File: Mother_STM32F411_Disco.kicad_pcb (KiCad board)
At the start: 2 copper layers, 200 x 200 mm, 38 parts, among them J1 SRC_Cable, J2 0, J3 0, J4 0, U1 ESP32-DEVKIT-V1

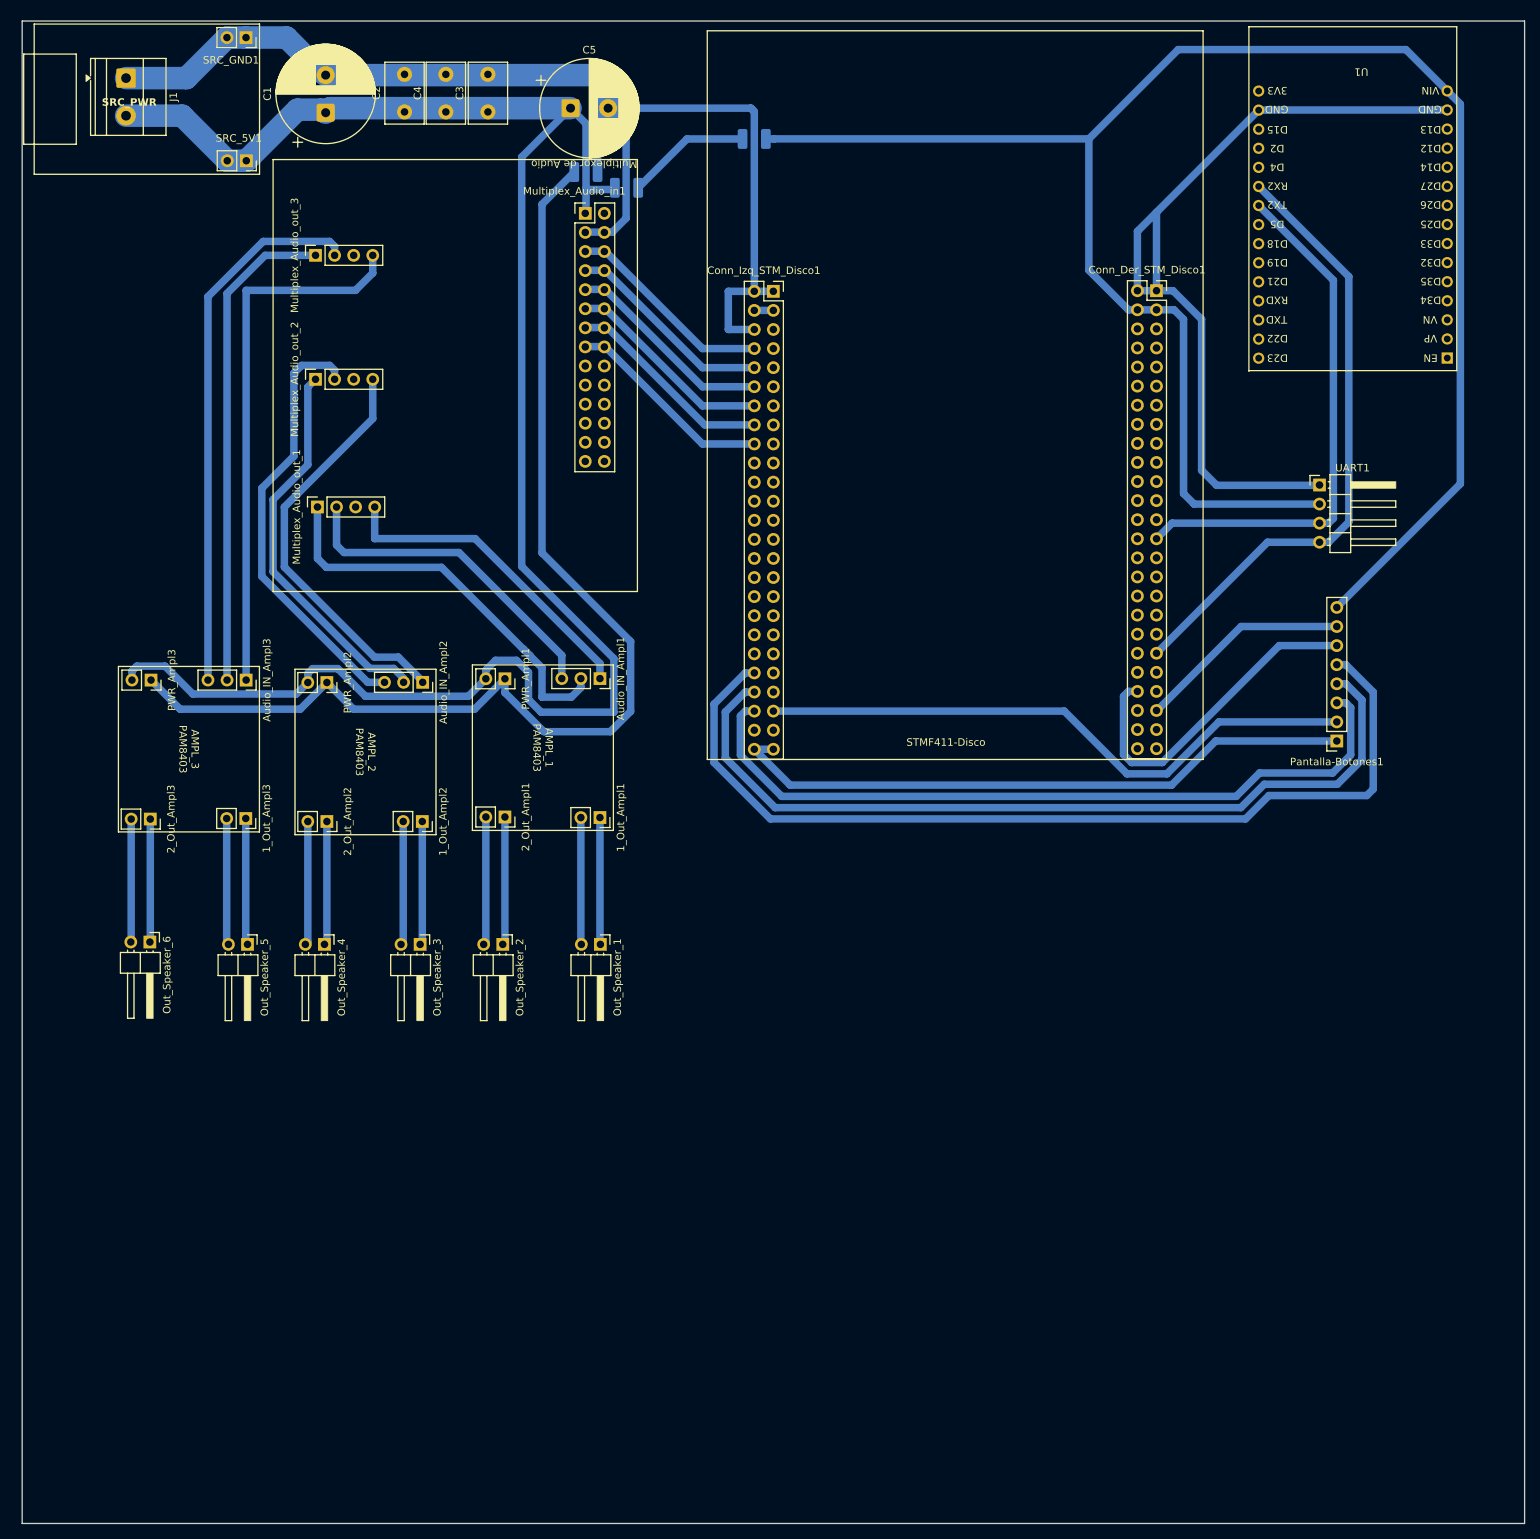
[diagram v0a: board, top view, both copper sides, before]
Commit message: PCB version 2
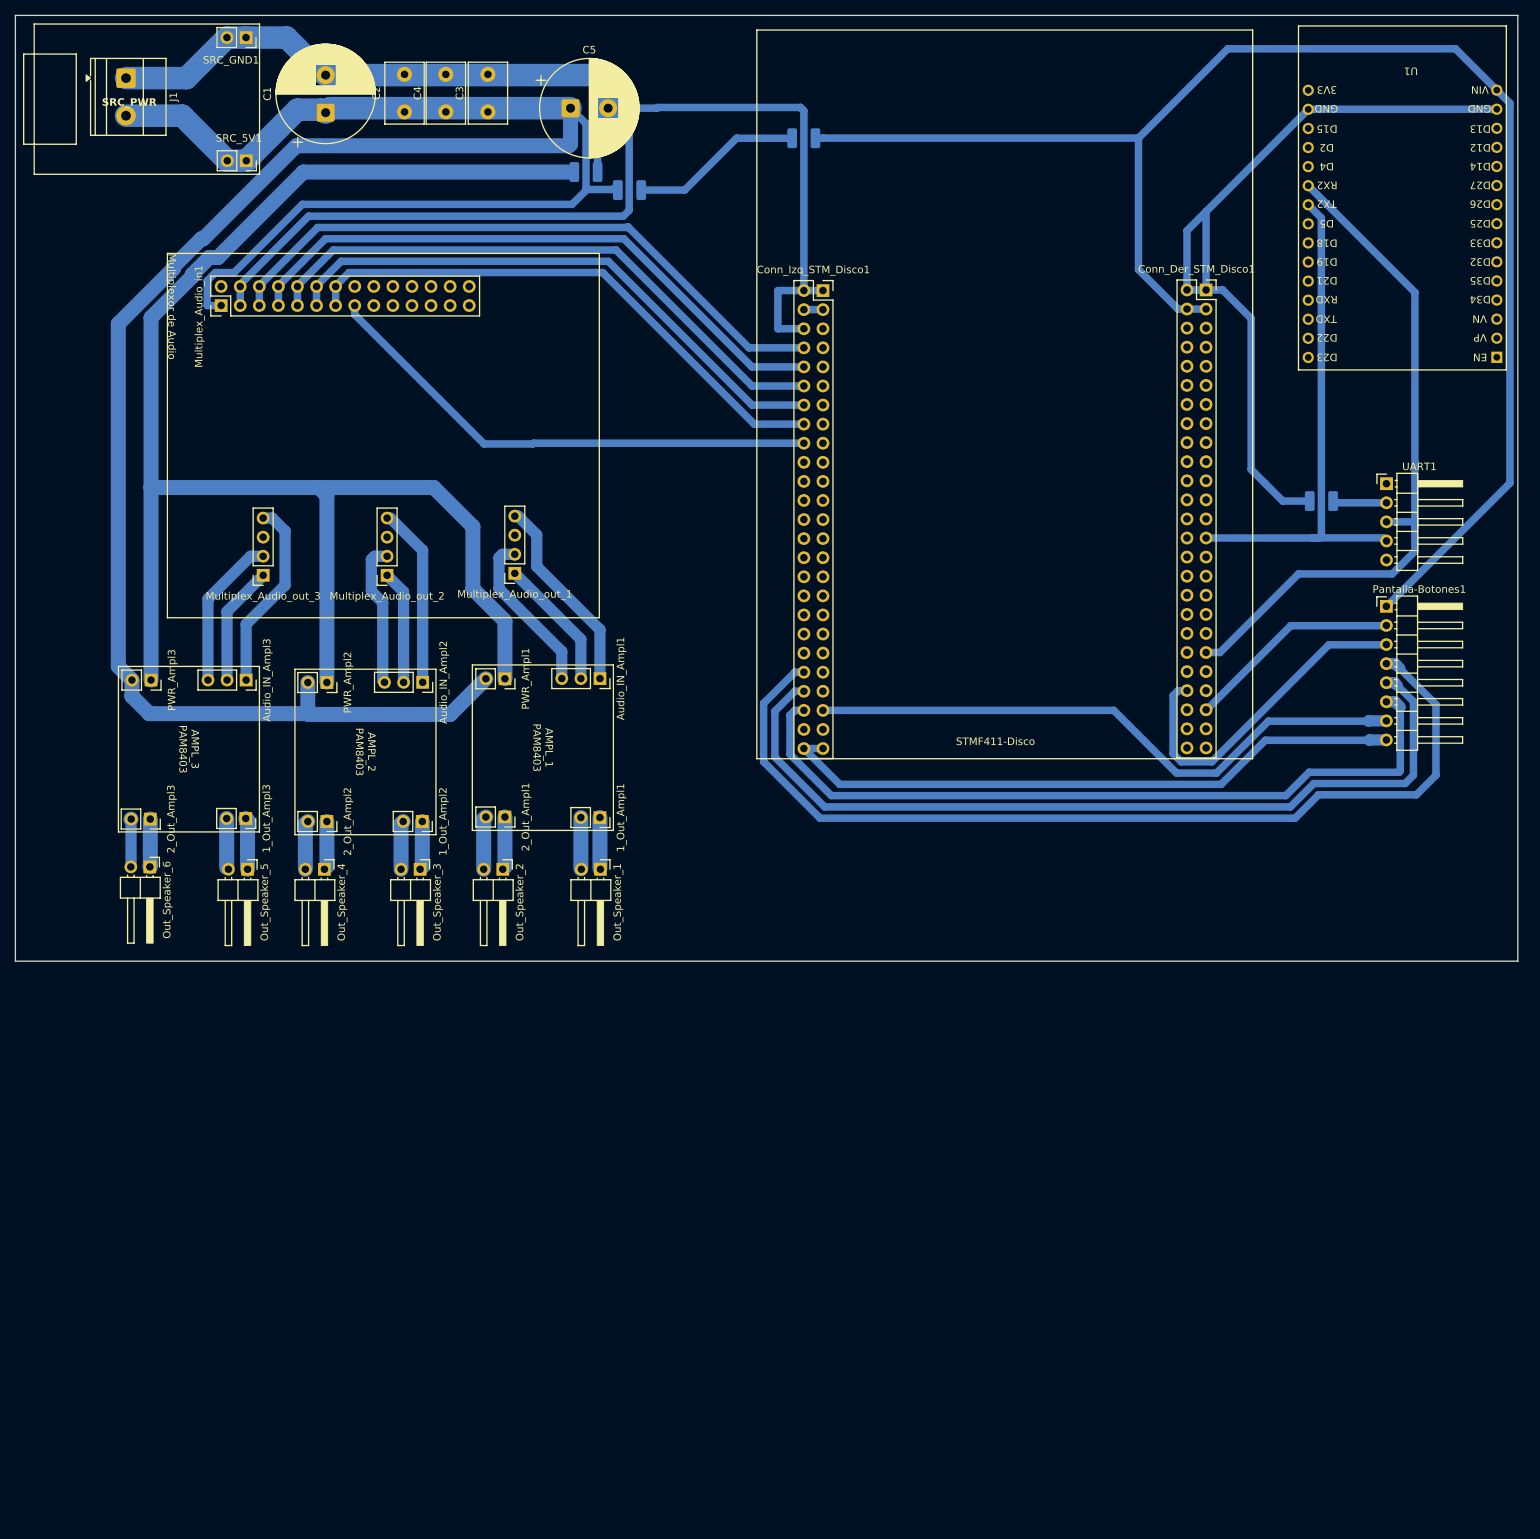
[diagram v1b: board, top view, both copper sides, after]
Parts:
- added J5: 0, Resistor_SMD:R_1210_3225Metric_Pad1.30x2.65mm_HandSolder, B.Cu at (342.9, 91.3)
- Pantalla-Botones1: footprint Connector_PinSocket_2.54mm:PinSocket_1x08_P2.54mm_Vertical -> Connector_PinHeader_2.54mm:PinHeader_1x08_P2.54mm_Horizontal
- UART1: footprint Connector_PinHeader_2.54mm:PinHeader_1x04_P2.54mm_Horizontal -> Connector_PinHeader_2.54mm:PinHeader_1x05_P2.54mm_Horizontal
- moved Multiplex_Audio_in1 50.0 mm to (196.5, 65.3), turned to 90 degrees
- moved Multiplex_Audio_out_3 43.2 mm to (202.1, 101.2), turned to 180 degrees
- moved Multiplex_Audio_out_2 27.8 mm to (218.6, 101.2), turned to 180 degrees
- moved Multiplex_Audio_out_1 27.7 mm to (235.6, 100.9), turned to 180 degrees
- moved Pantalla-Botones1 19.1 mm to (351.6, 105.3), turned to 0 degrees
- moved Out_Speaker_1 10.0 mm to (247.0, 140.3)
- moved Out_Speaker_2 10.0 mm to (234.0, 140.3)
- moved Out_Speaker_3 10.0 mm to (223.0, 140.3)
- moved Out_Speaker_4 10.0 mm to (210.2, 140.3)
- moved Out_Speaker_5 10.0 mm to (200.0, 140.3)
- moved Out_Speaker_6 10.0 mm to (187.0, 140.0)
- moved UART1 8.92 mm to (351.6, 89.0)
- moved Conn_Der_STM_Disco1 6.60 mm to (327.6, 63.2)
- moved Conn_Izq_STM_Disco1 6.60 mm to (276.6, 63.3)
- moved J2 6.60 mm to (274.1, 43.0)
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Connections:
- Pantalla-Botones1 pad 1: /GND -> /5V
- Pantalla-Botones1 pad 2: /PD14 -> /PC9
- Pantalla-Botones1 pad 3: /PD13 -> /PA8
- Pantalla-Botones1 pad 4: /PD11 -> /PD9
- Pantalla-Botones1 pad 5: /PD9 -> /PD11
- Pantalla-Botones1 pad 6: /PA8 -> /PD13
- Pantalla-Botones1 pad 7: /PC9 -> /PD14
- Pantalla-Botones1 pad 8: /5V -> /GND
- UART1 pad 1: /GND -> /5V
- UART1 pad 2: /5V -> Net-(UART1-Pin_2)
- UART1 pad 3: /PB3 -> /PA15
- UART1 pad 4: /PA15 -> /PB3
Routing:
- net /5V: track 515.3 -> 577.6 mm
- net /PC1: track 27.8 -> 85.0 mm
- net /PC3: track 27.8 -> 82.2 mm
- net /GND: track 358.7 -> 412.4 mm
- net /GND_Analg: track 153.6 -> 205.7 mm
- net Net-(Audio_IN_Ampl3-Pin_3): track 72.4 -> 20.5 mm
- net /PA1: track 27.8 -> 79.6 mm
- net Net-(Audio_IN_Ampl3-Pin_2): track 65.3 -> 15.9 mm
- net /PA3: track 27.8 -> 76.8 mm
- net Net-(Audio_IN_Ampl3-Pin_1): track 72.1 -> 25.6 mm
- net /PA5: track 27.8 -> 74.0 mm
- net /PA7: track 27.8 -> 68.2 mm
- net Net-(Audio_IN_Ampl2-Pin_3): track 58.3 -> 19.4 mm
- net Net-(Audio_IN_Ampl2-Pin_2): track 51.7 -> 15.2 mm
- net Net-(Audio_IN_Ampl1-Pin_2): track 53.6 -> 17.6 mm
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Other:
- board size 200 x 200 mm -> 200 x 125.9 mm
